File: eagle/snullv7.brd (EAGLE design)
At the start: 33 parts, among them X1 MKDSN1,5/6-5,08, X2 MKDSN1,5/6-5,08

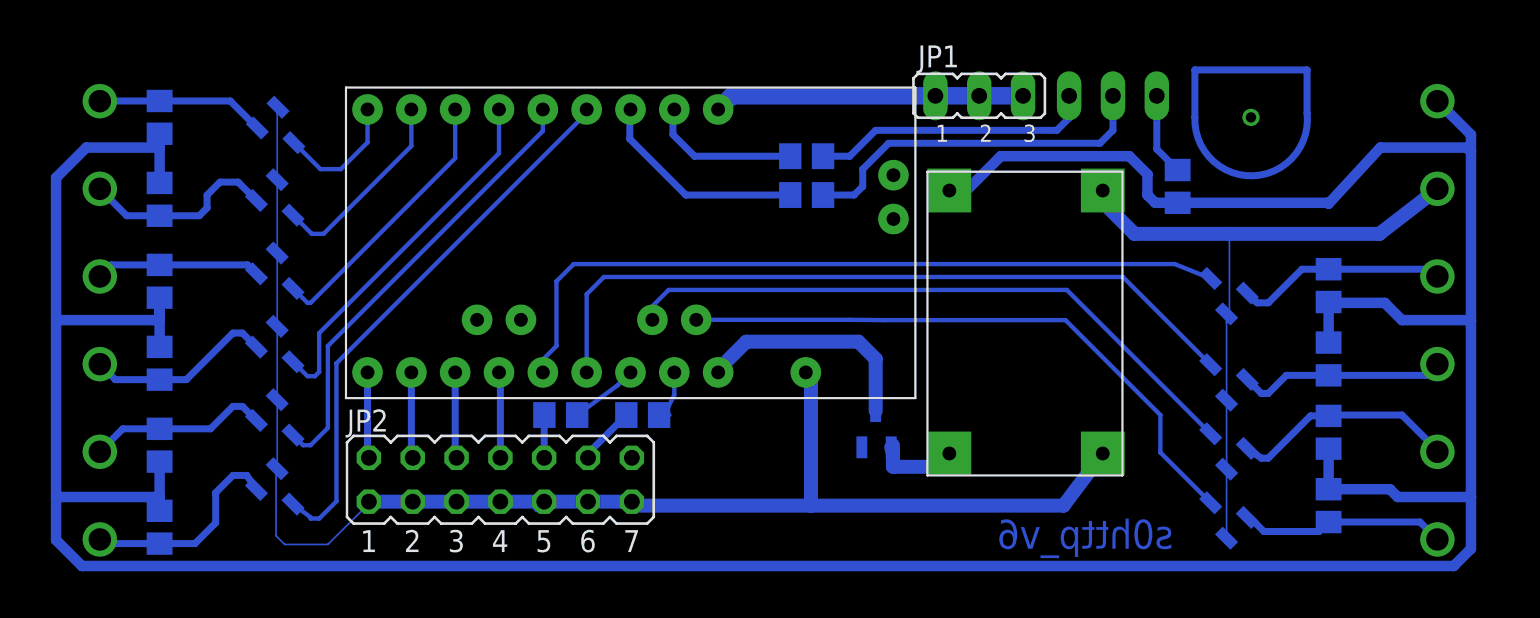
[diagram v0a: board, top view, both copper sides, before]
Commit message: added v8, added stiker, updated pinning in sketch
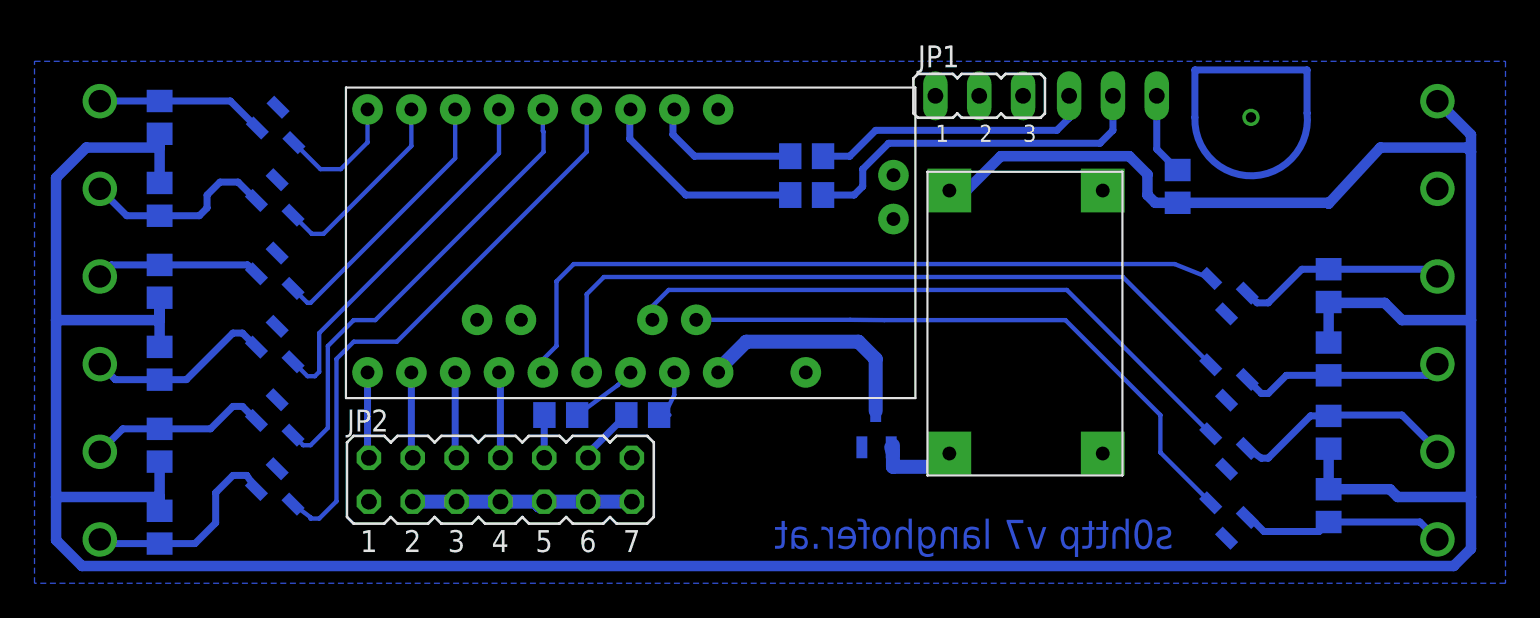
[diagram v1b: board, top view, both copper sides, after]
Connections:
- removed net N$31: JP2.1, JP2.11, JP2.13, JP2.3, JP2.5, JP2.7, JP2.9, U$1.GND2, U$2.GNDOUT, U$3.S, U$4.S, U$5.S, U$6.S, U$7.S, U$8.S
- removed net N$32: JP1.1, JP1.2, JP1.3, U$1.GND1
- removed net VDD: U$10.S, U$11.S, U$12.S, U$2.GNDIN, U$9.S, X2.5
- new net GND: JP1.1, JP1.2, JP1.3, JP2.1, JP2.11, JP2.13, JP2.3, JP2.5, JP2.7, JP2.9, U$1.GND1, U$1.GND2, U$10.S, U$11.S, U$12.S, U$2.GNDIN, U$2.GNDOUT, U$3.S, U$4.S, U$5.S, U$6.S, U$7.S, U$8.S, U$9.S, X2.5
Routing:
- net N$31: track 84.4 -> 0.00 mm
- net VDD: track 40.3 -> 0.00 mm
- net N$32: track 18.0 -> 0.00 mm
- net GND: track 0.00 -> 13.5 mm
- net N$17: track 32.0 -> 33.4 mm
- net N$15: track 26.3 -> 27.1 mm
- added copper zone on layer 16, net GND
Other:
- board text added: "s0http v7 langhofer.at"
- board text removed: "s0http_v6"
